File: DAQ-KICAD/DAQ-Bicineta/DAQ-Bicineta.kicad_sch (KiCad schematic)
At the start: 10 parts, among them J1 Conn_01x02, U3 ESP32-DEVKIT-V1

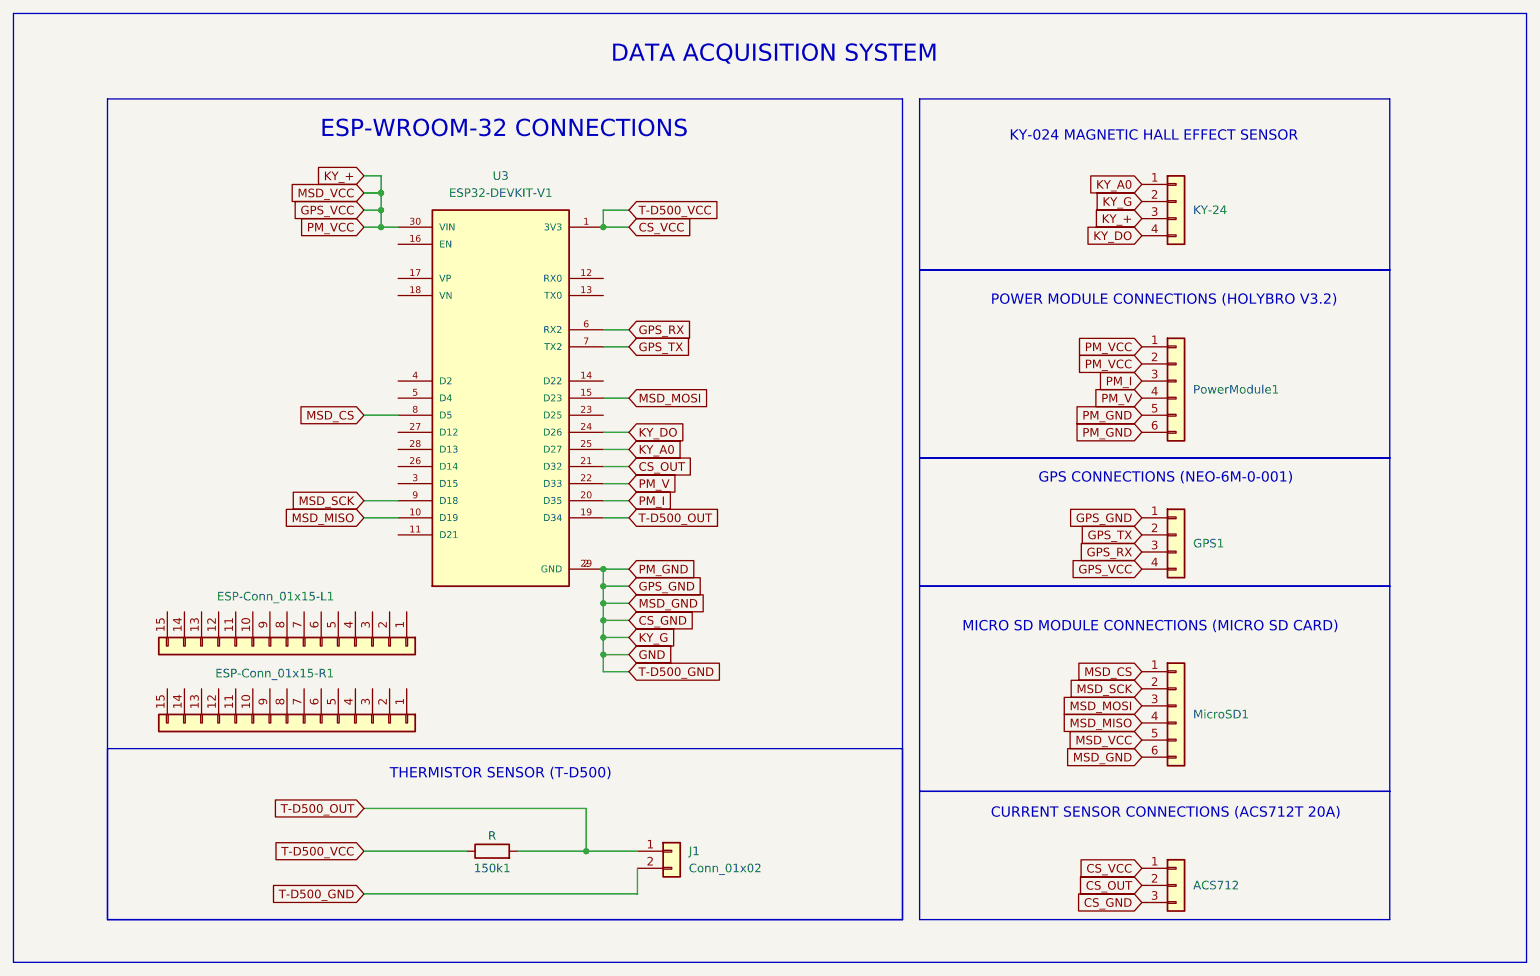
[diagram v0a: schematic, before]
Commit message: DAQ-V2-KICAD-modification
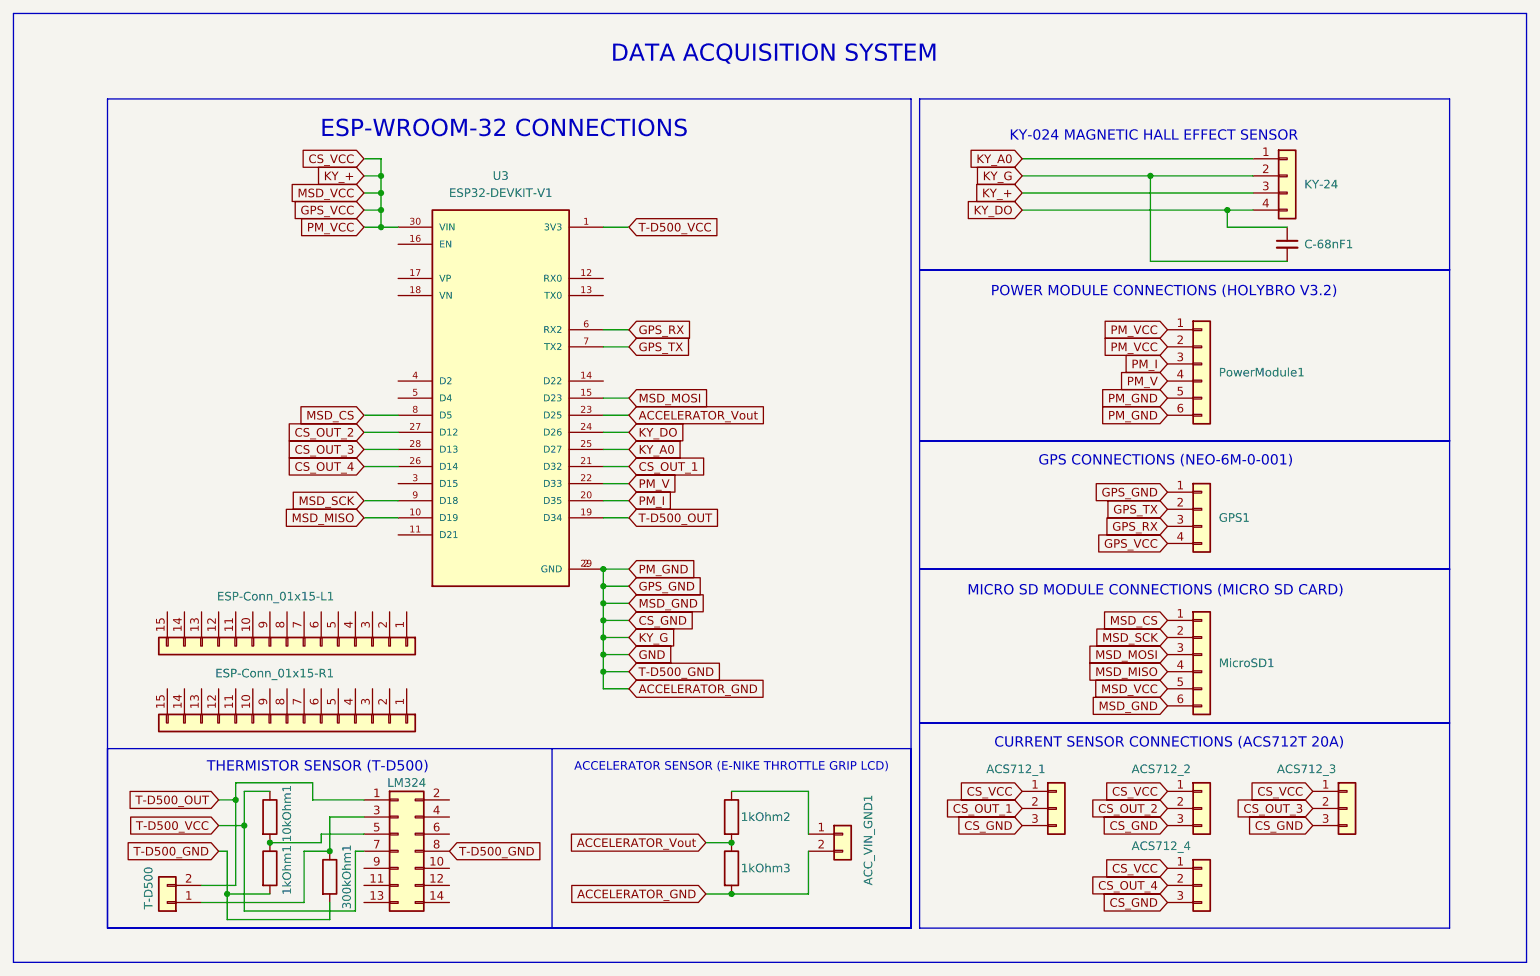
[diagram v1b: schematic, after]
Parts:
- added 10kOhm1, 1kOhm1, 1kOhm2, 1kOhm3: R, Connector_PinSocket_2.54mm:PinSocket_1x02_P2.54mm_Vertical, symbol Device:R
- added ACC_VIN_GND1: Conn_01x02, Connector_PinSocket_2.54mm:PinSocket_1x02_P2.54mm_Vertical, symbol Connector_Generic:Conn_01x02
- added ACS712_2, ACS712_3, ACS712_4: Conn_01x03, Connector_PinSocket_2.54mm:PinSocket_1x03_P2.54mm_Vertical, symbol Connector_Generic:Conn_01x03
- added C-68nF1: C_Small, Connector_PinSocket_2.54mm:PinSocket_1x02_P2.54mm_Vertical, symbol Device:C_Small
- added LM324: Conn_02x07_Odd_Even, MyPrintFoot:LM324, symbol Connector_Generic:Conn_02x07_Odd_Even
- KY-24: footprint Connector_PinSocket_2.54mm:PinSocket_1x04_P2.54mm_Horizontal -> Connector_PinSocket_2.54mm:PinSocket_1x04_P2.54mm_Vertical
- MicroSD1: footprint Connector_PinSocket_2.54mm:PinSocket_1x06_P2.54mm_Horizontal -> Connector_PinSocket_2.54mm:PinSocket_1x06_P2.54mm_Vertical
- renumbered 150k1 to 300kOhm1, ACS712 to ACS712_1, J1 to T-D500
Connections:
- net GPS_VCC is gone; now on net CS_VCC: GPS1.4 (Pin_4), KY-24.3 (Pin_3), MicroSD1.5 (Pin_5), PowerModule1.1 (Pin_1), PowerModule1.2 (Pin_2), U3.30 (VIN)
- net CS_VCC: now also ACS712_2.1 (Pin_1), ACS712_3.1 (Pin_1), ACS712_4.1 (Pin_1); no longer 300kOhm1.1, U3.1 (3V3)
- net KY_DO: now also C-68nF1.1
- net T-D500_OUT: now also T-D500.2 (Pin_2), LM324.1 (Pin_1); no longer 300kOhm1.2, T-D500.1 (Pin_1)
- net ACCELERATOR_Vout: now reaches U3.23 (D25)
- net ACCELERATOR_Vout: now also 1kOhm2.2, 1kOhm3.1
- net CS_OUT_4: now reaches U3.26 (D14)
- net CS_OUT_4: now also ACS712_4.2 (Pin_2)
- net CS_OUT_2: now reaches U3.27 (D12)
- net CS_OUT_2: now also ACS712_2.2 (Pin_2)
- net CS_OUT_3: now reaches U3.28 (D13)
- net CS_OUT_3: now also ACS712_3.2 (Pin_2)
- net CS_GND renamed ACCELERATOR_GND
- net ACCELERATOR_GND: now also 300kOhm1.2, 1kOhm1.2, 1kOhm3.2, ACC_VIN_GND1.2 (Pin_2), ACS712_2.3 (Pin_3), ACS712_3.3 (Pin_3), ACS712_4.3 (Pin_3), C-68nF1.2, LM324.8 (Pin_8); no longer T-D500.2 (Pin_2)
- net CS_OUT renamed CS_OUT_1
- new net: 300kOhm1.1, LM324.3 (Pin_3), T-D500.1 (Pin_1)
- new net: 1kOhm2.1, ACC_VIN_GND1.1 (Pin_1)
- new net: 10kOhm1.2, 1kOhm1.1, LM324.5 (Pin_5)
- new net T-D500_VCC: 10kOhm1.1, LM324.7 (Pin_7), U3.1 (3V3)
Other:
- note added: "ACCELERATOR SENSOR (E-NIKE THROTTLE GRIP LCD)"
- moved on the sheet: 300kOhm1, ACS712_1, GPS1, KY-24, MicroSD1, PowerModule1, T-D500
